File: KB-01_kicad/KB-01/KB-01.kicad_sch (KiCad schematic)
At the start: 2 parts

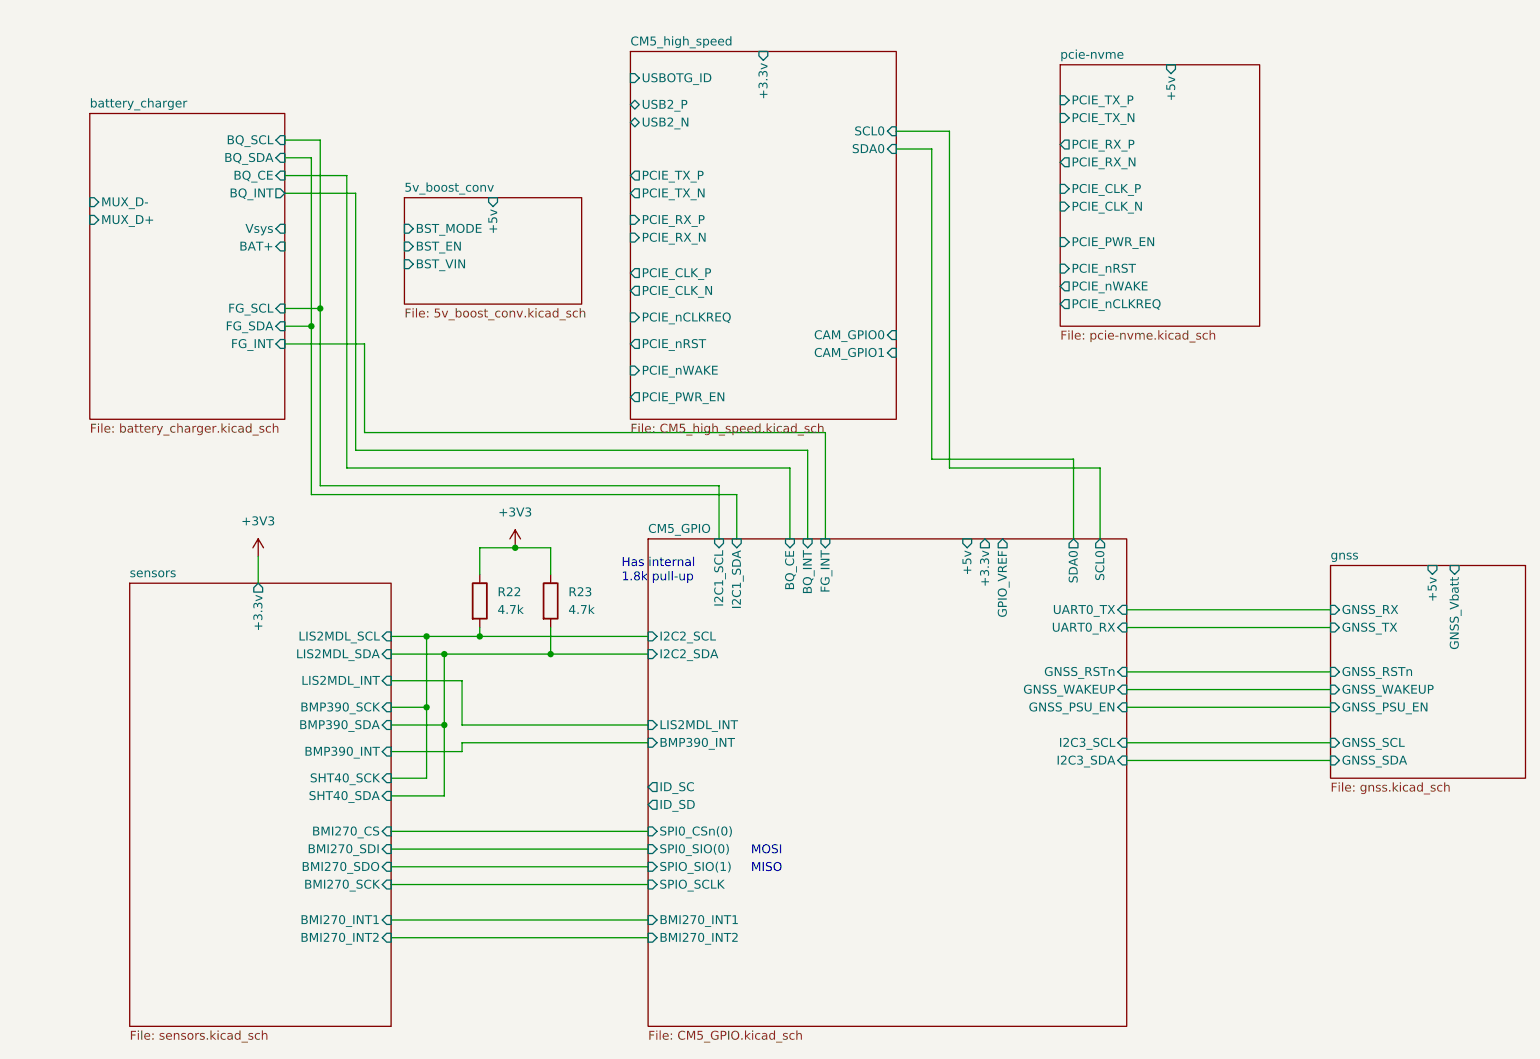
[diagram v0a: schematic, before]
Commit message: all
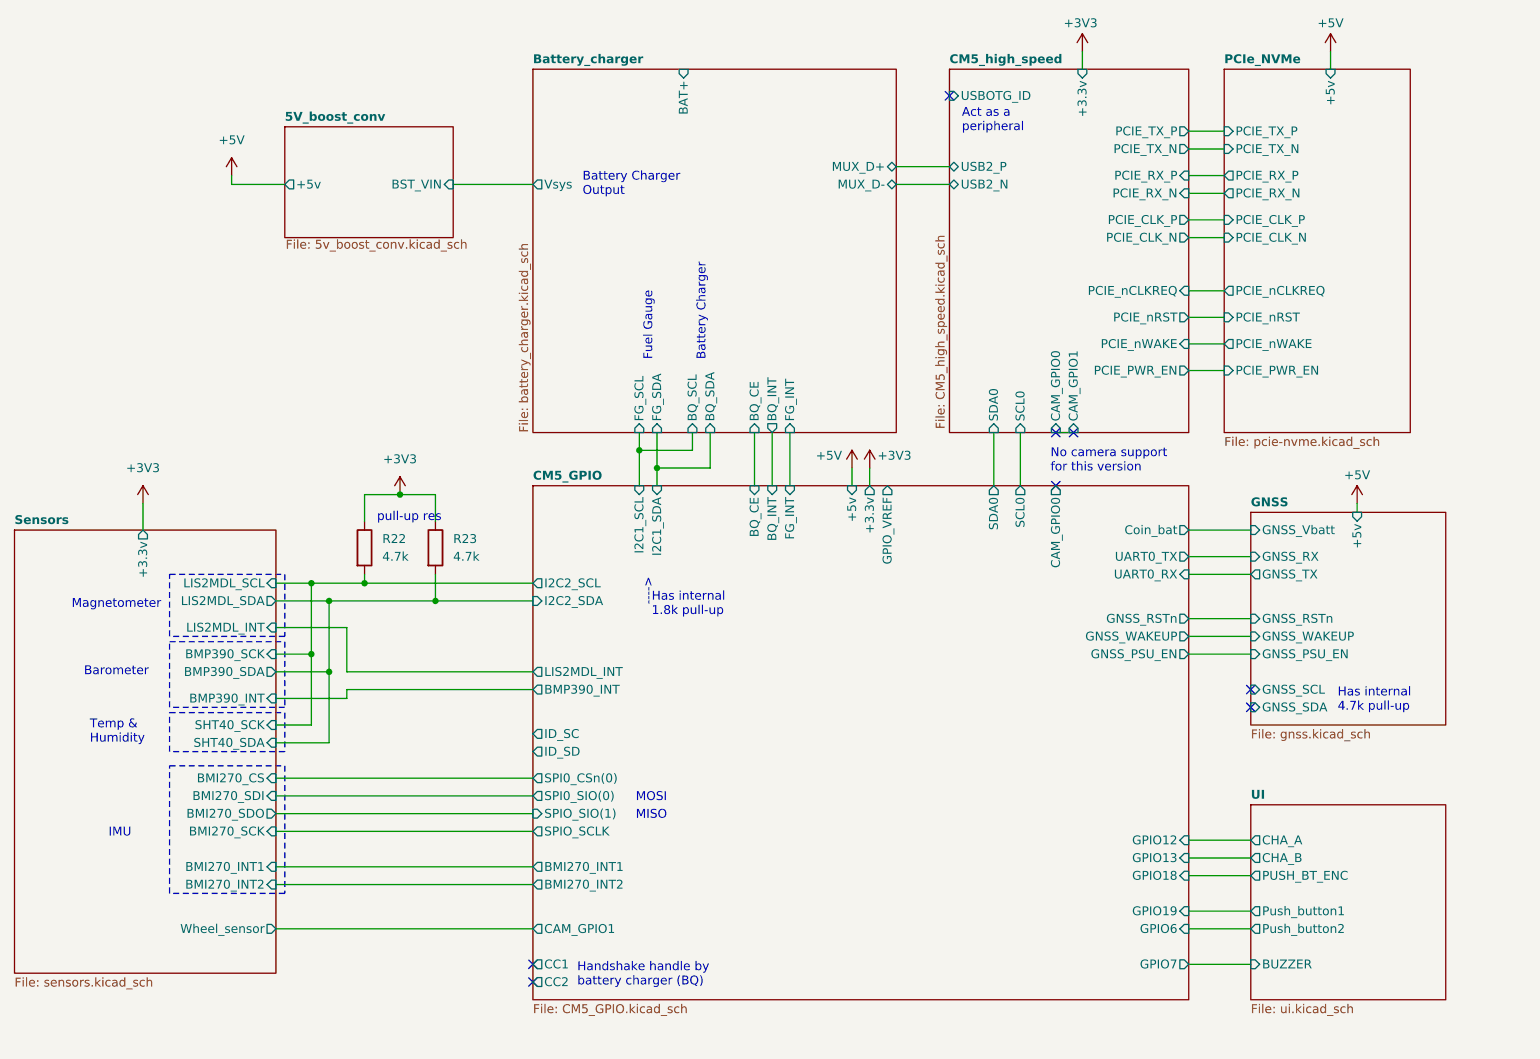
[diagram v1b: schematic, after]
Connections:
- no-connect marks 0 -> 8
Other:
- sheet 5v_boost_conv renamed 5V_boost_conv
- sheet battery_charger renamed Battery_charger
- sheet gnss renamed GNSS
- sheet pcie-nvme renamed PCIe_NVMe
- sheet sensors renamed Sensors
- added sheet UI (ui.kicad_sch)
- sheet 5V_boost_conv ports: added none; removed BST_EN, BST_MODE
- sheet CM5_GPIO ports: added CAM_GPIO0, CAM_GPIO1, CC1, CC2, Coin_bat, GPIO12, GPIO13, GPIO18, GPIO19, GPIO6, GPIO7; removed I2C3_SCL, I2C3_SDA
- sheet Sensors ports: added Wheel_sensor; removed none
- note added: "---->"
- note added: "Act as a peripheral"
- note added: "Barometer"
- note added: "Battery Charger"
- note added: "Battery Charger Output"
- note added: "Fuel Gauge"
- note added: "Handshake handle by battery charger (BQ)"
- note added: "Has internal 4.7k pull-up"
- note added: "IMU"
- note added: "Magnetometer"
- note added: "No camera support for this version"
- note added: "Temp & Humidity"
- note added: "pull-up res"
- company: (none) -> Otai Labs
- title: (none) -> Komputer Basikal, KB-01
- moved on the sheet: R22, R23
